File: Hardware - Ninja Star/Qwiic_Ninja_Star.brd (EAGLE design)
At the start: 40.6 x 40.6 mm, 30 parts, among them J1 QWIIC_RIGHT_ANGLE, J2 QWIIC_RIGHT_ANGLE, J3 QWIIC_RIGHT_ANGLE, J4 QWIIC_RIGHT_ANGLE

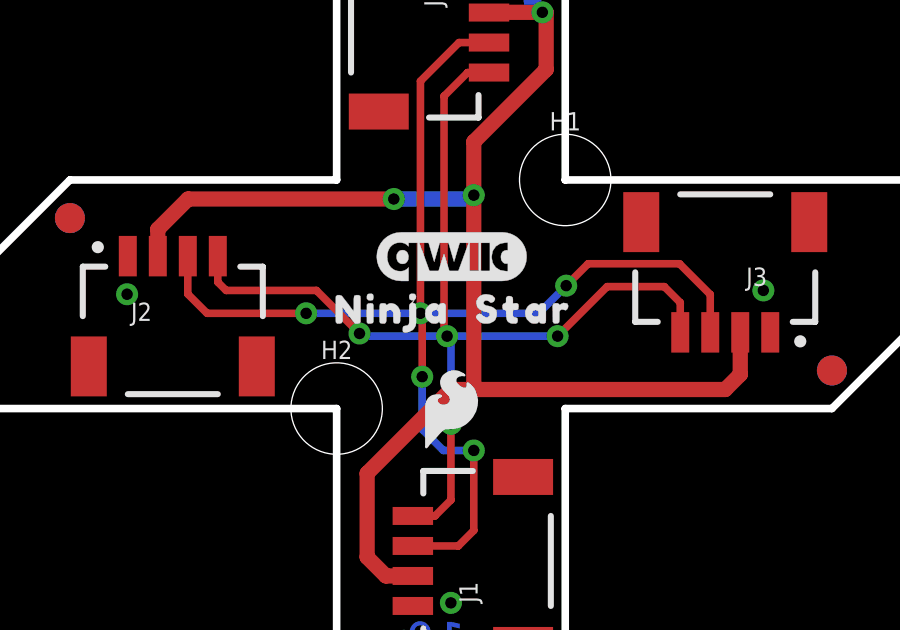
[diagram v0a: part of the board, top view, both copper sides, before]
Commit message: Completed Engineering checklist
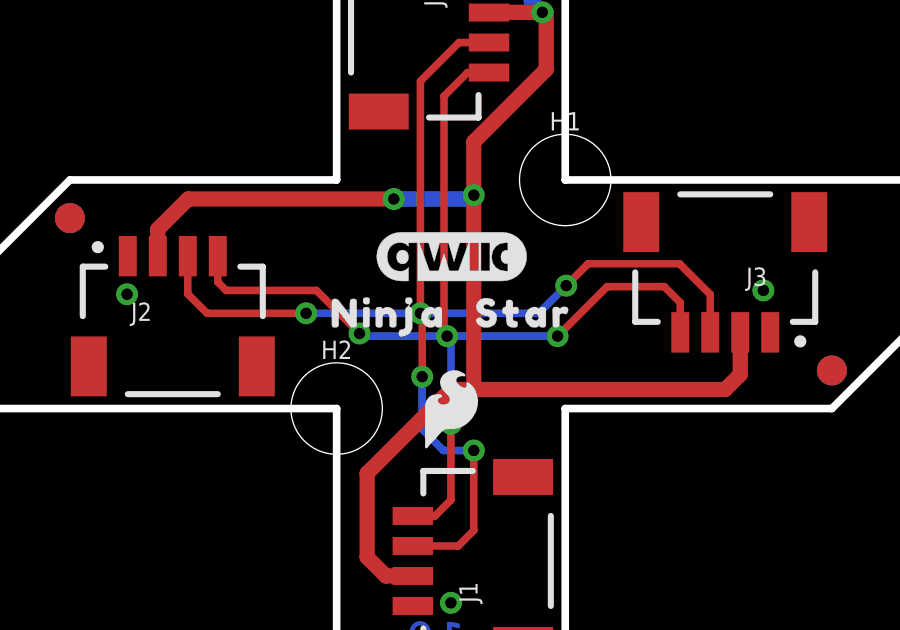
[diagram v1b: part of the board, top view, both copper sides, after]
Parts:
- moved U$3 0.18 mm to (15.6, 19.7)
- moved U$6 0.13 mm to (20.4, 19.7)
- moved U$5 0.13 mm to (22.9, 12.2)
- moved U$7 0.13 mm to (22.5, 10.8)
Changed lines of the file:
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@@
 <?xml version="1.0" encoding="utf-8"?>
 <!DOCTYPE eagle SYSTEM "eagle.dtd">
-<eagle version="9.6.2">
+<eagle version="9.5.2">
 <drawing>
 <settings>
-<setting alwaysvectorfont="no"/>
+<setting alwaysvectorfont="yes"/>
 <setting verticaltext="up"/>
 </settings>
@@
 <layer number="37" name="tTest" color="7" fill="1" visible="no" active="yes"/>
 <layer number="38" name="bTest" color="7" fill="1" visible="no" active="yes"/>
-<layer number="39" name="tKeepout" color="4" fill="11" visible="yes" active="yes"/>
+<layer number="39" name="tKeepout" color="4" fill="11" visible="no" active="yes"/>
 <layer number="40" name="bKeepout" color="1" fill="11" visible="no" active="yes"/>
-<layer number="41" name="tRestrict" color="4" fill="10" visible="yes" active="yes"/>
+<layer number="41" name="tRestrict" color="4" fill="10" visible="no" active="yes"/>
 <layer number="42" name="bRestrict" color="1" fill="10" visible="no" active="yes"/>
 <layer number="43" name="vRestrict" color="2" fill="10" visible="no" active="yes"/>
@@
 <element name="LOGO8" library="SparkFun-Aesthetics" package="SFE_LOGO_FLAME_.1" value="SFE_LOGO_FLAME.1_INCH" x="3.429" y="18.161" smashed="yes" rot="MR90"/>
 <element name="U$1" library="SparkFun-Aesthetics" package="ORDERING_INSTRUCTIONS" value="" x="44.45" y="50.8" smashed="yes"/>
-<element name="U$3" library="output" package="NINJA0" value="" x="15.748" y="19.812" smashed="yes"/>
-<element name="U$5" library="output" package="NINJA0" value="" x="22.86" y="12.065" smashed="yes" rot="MR0"/>
-<element name="U$6" library="output" package="STAR0" value="" x="20.447" y="19.812" smashed="yes"/>
-<element name="U$7" library="output" package="STAR0" value="" x="22.479" y="10.668" smashed="yes" rot="MR0"/>
+<element name="U$3" library="output" package="NINJA0" value="" x="15.621" y="19.685" smashed="yes"/>
+<element name="U$5" library="output" package="NINJA0" value="" x="22.86" y="12.192" smashed="yes" rot="MR0"/>
+<element name="U$6" library="output" package="STAR0" value="" x="20.447" y="19.685" smashed="yes"/>
+<element name="U$7" library="output" package="STAR0" value="" x="22.479" y="10.795" smashed="yes" rot="MR0"/>
 </elements>
 <signals>
